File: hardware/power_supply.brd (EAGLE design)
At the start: 76.2 x 38.1 mm, 33 parts, among them Q1 IRF630N, U1 MC34063, U2 AP1507

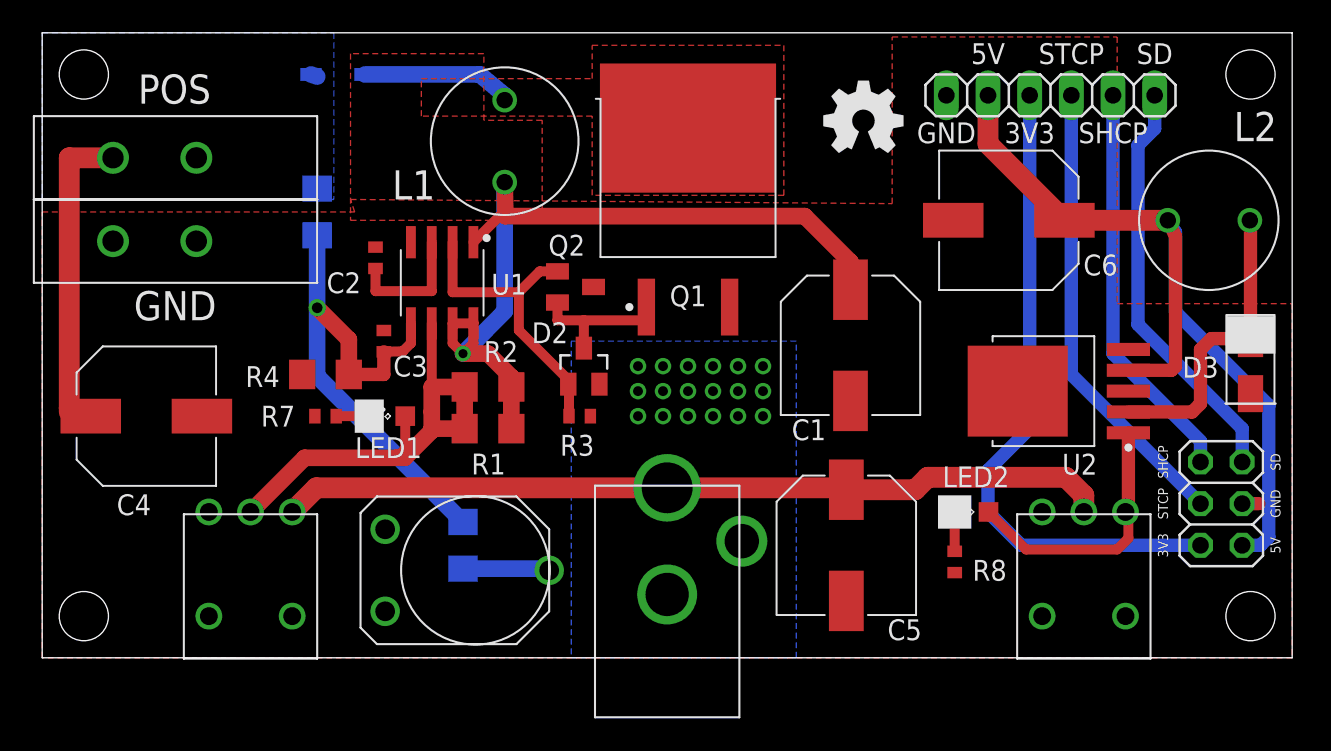
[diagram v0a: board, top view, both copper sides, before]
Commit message: Updating power_supply
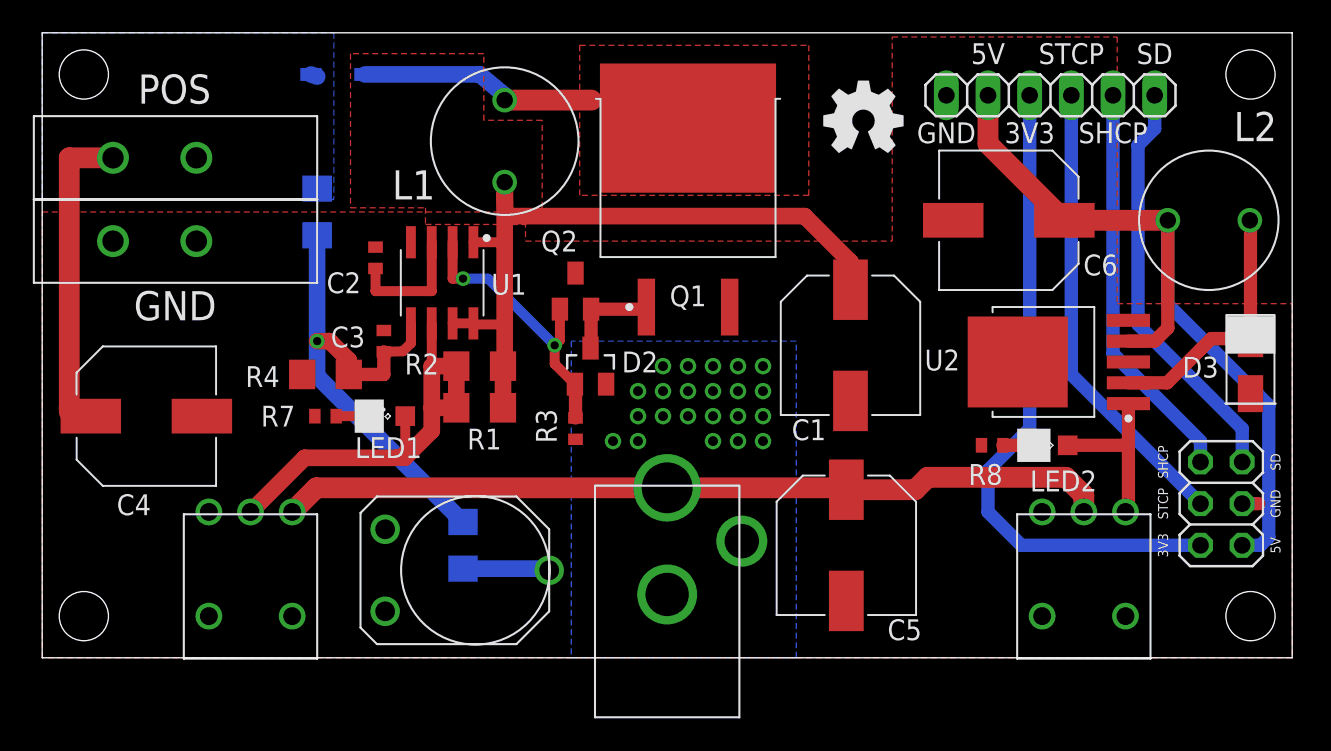
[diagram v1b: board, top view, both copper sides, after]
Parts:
- moved R8 7.47 mm to (57.9, 13.0), turned to 0 degrees
- moved LED2 6.31 mm to (61.5, 13.0)
- moved U2 1.78 mm to (62.0, 18.0)
- moved R1 1.37 mm to (26.7, 15.2)
- moved R2 1.37 mm to (26.7, 17.8)
- moved R3 0.80 mm to (32.5, 14.0), turned to 90 degrees
- moved D2 0.41 mm to (33.4, 17.8)
- moved Q2 0.25 mm to (32.5, 22.4), turned to 0 degrees
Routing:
- net N$1: track 53.2 -> 45.3 mm, vias 1 -> 0
- net N$8: track 16.4 -> 10.4 mm
- net N$2: track 9.26 -> 14.6 mm
- net N$10: track 18.4 -> 15.8 mm
- net +5V: track 51.5 -> 48.8 mm
- net N$6: track 30.5 -> 27.9 mm
- net N$5: track 9.09 -> 6.63 mm
- net N$9: track 32.6 -> 31.0 mm
- net N$4: track 18.8 -> 17.4 mm, vias 0 -> 2
- net N$12: track 2.41 -> 1.86 mm
- net GND: vias 18 -> 22

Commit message: Updating 8-12
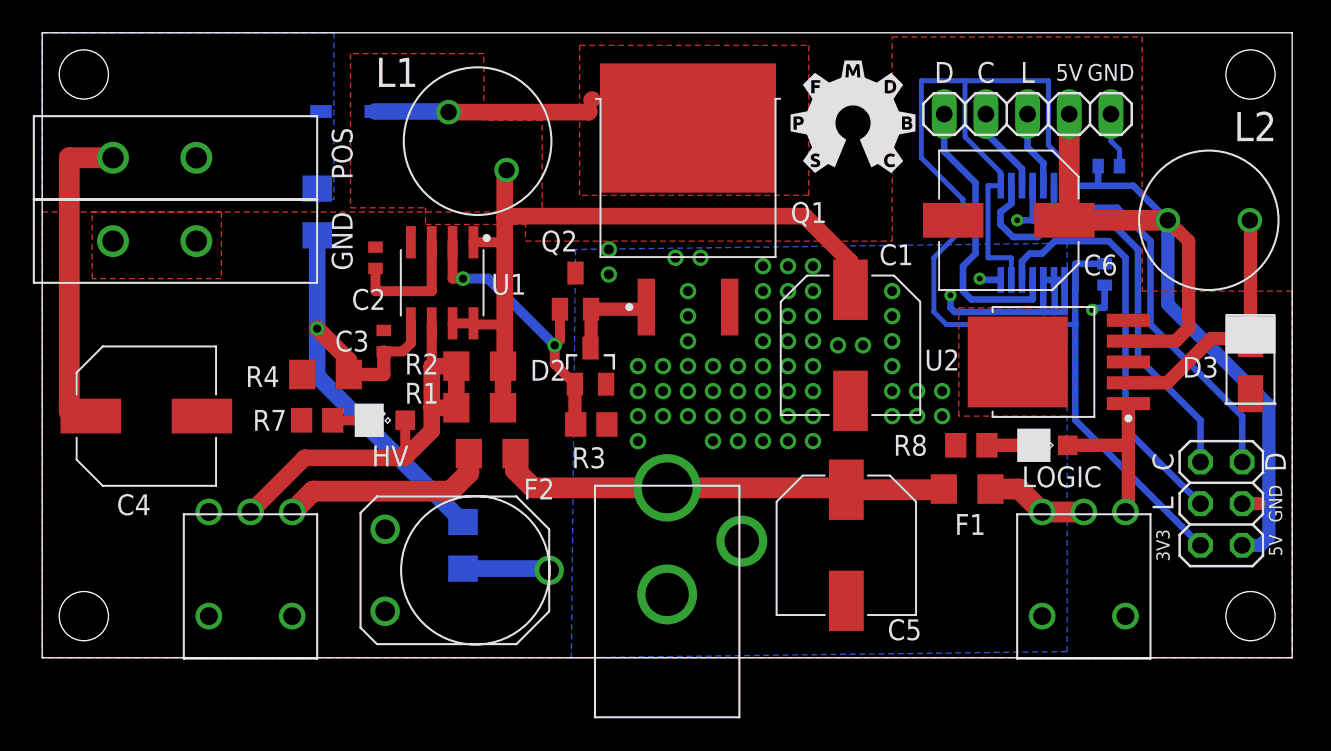
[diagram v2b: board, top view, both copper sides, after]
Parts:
- removed JP1: (no value), pinhead:1X06
- removed LED1: (no value), led:SML0805
- added C7, C8: (no value), resistor:C0402
- added F1, F2: FUSE_1206, nixie_ticker:R1206
- added HV: (no value), led:SML0805
- added JP3: (no value), pinhead:1X05
- added U3: CD40109B_SPLITEN, nixie_ticker:SOP65P640X120-16
- C1, C5, C6: value UUR1C221MCL6GS -> 220uF
- C2: value (none) -> 680pF
- C3: value (none) -> 0.01uF
- C4: value UUR1C221MCL6GS -> 3.3uF
- D1: value BAV21W -> (none)
- D2: value MMBD914L -> (none)
- L1: value RLB9012 -> 100uH
- R3: device resistor:R0402 -> resistor:R0805
- R7, R8: value 1k -> 2k; device resistor:R0402 -> resistor:R0805
- RX: value 3309P-1-202 -> 2k
- moved D1 2.34 mm to (18.6, 33.3)
- moved L1 1.65 mm to (26.5, 31.5), turned to 225 degrees
- moved R8 1.27 mm to (56.6, 13.0)
- moved R3 1.00 mm to (33.5, 14.2), turned to 180 degrees
- moved R7 0.57 mm to (16.8, 14.5)
- renumbered LED2 to LOGIC, U$2 to RX, U$3 to SW1, U$4 to SW2, U$9 to L2
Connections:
- removed net DI: JP1.6, JP2.2
- removed net SHCP: JP1.5, JP2.1
- removed net STCP: JP1.4, JP2.3
- new net CLK_H: JP3.4, U3.11
- new net CLK_L: JP2.1, U3.10
- new net DATA_H: JP3.5, U3.5
- new net DATA_L: JP2.2, U3.14
- new net LATCH_H: JP3.3, U3.13
- new net LATCH_L: JP2.3, U3.6
- new net N$13: F1.2, SW2.P$2, SW2.P$3
- new net N$14: F2.2, SW1.P$1
- net +12V: now also F1.1, F2.1; no longer SW1.P$1, SW2.P$2
- net +3V3: now also C7.1, U3.1, U3.15, U3.7, U3.9; no longer JP1.3
- net +5V: now also C8.1, JP3.2, U3.16; no longer JP1.2
- net GND: now also C7.2, C8.2, JP3.1, U3.12, U3.2, U3.3, U3.4, U3.8; no longer JP1.1
- net N$11: now also HV.C; no longer LED1.C
- net N$6: now also HV.A; no longer LED1.A
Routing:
- net +3V3: track 40.2 -> 76.8 mm
- net STCP: track 28.2 -> 0.00 mm
- net CLK_L: track 0.00 -> 26.9 mm
- net GND: track 1.02 -> 27.5 mm, vias 22 -> 65
- net DI: track 25.4 -> 0.00 mm
- net LATCH_L: track 0.00 -> 25.3 mm
- net SHCP: track 24.6 -> 0.00 mm
- net DATA_L: track 0.00 -> 23.8 mm
- net +12V: track 50.7 -> 27.6 mm
- net DATA_H: track 0.00 -> 17.5 mm
- net N$14: track 0.00 -> 12.9 mm
- net +5V: track 48.8 -> 55.5 mm
- net N$13: track 0.00 -> 6.27 mm
- net CLK_H: track 0.00 -> 5.28 mm
- net LATCH_H: track 0.00 -> 4.76 mm
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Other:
- board text added: "C"
- board text added: "D"
- board text added: "L"
- board text removed: "SD"
- board text removed: "SHCP"
- board text removed: "STCP"
